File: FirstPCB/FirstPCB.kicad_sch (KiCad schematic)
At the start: 18 parts, among them J1 Conn_01x04_Socket, J2 Conn_01x08_Socket, U1 STM32G0B1KETx, U2 AMS1117-3.3

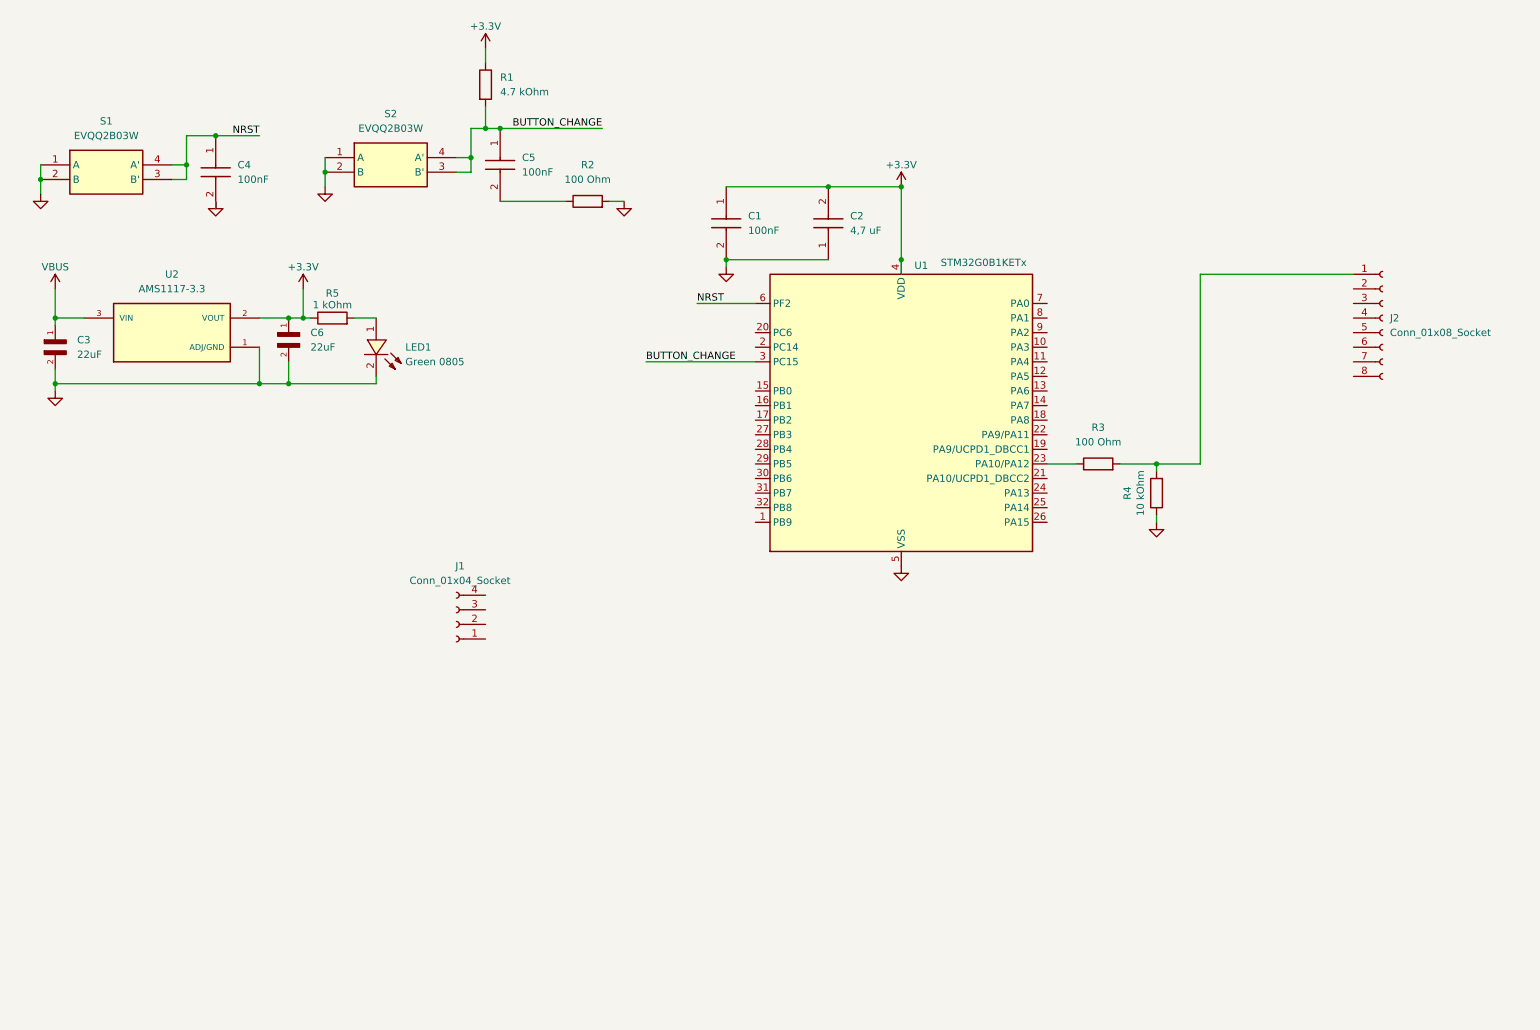
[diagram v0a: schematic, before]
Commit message: added sensor and schematic update
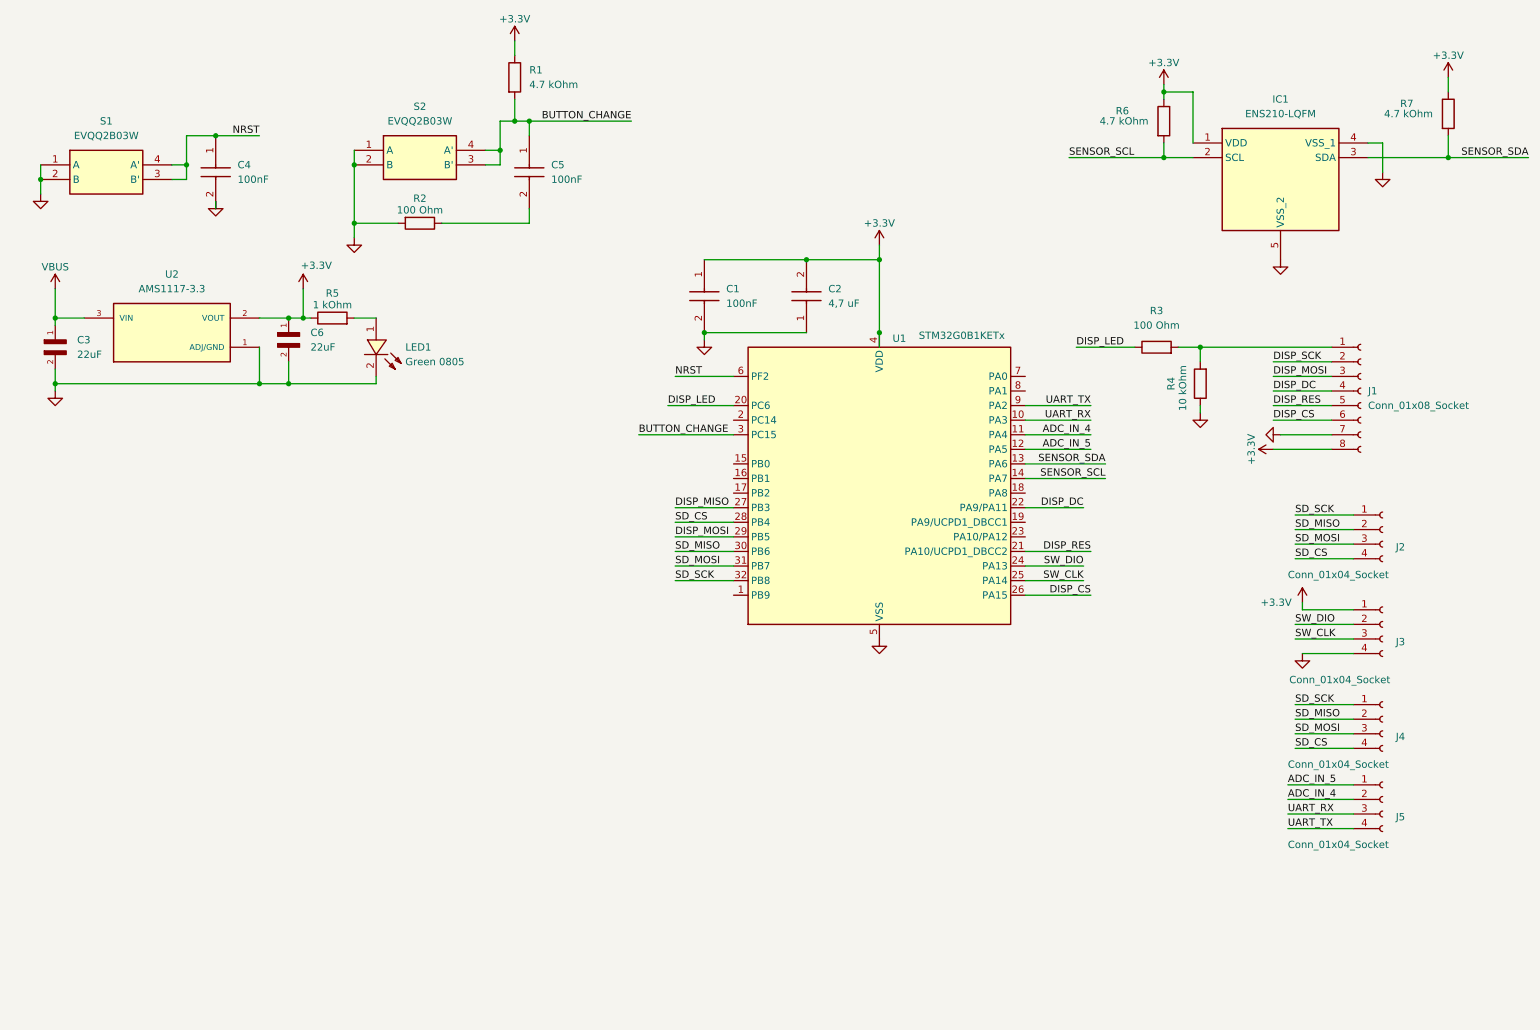
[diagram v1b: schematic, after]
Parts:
- added IC1: ENS210-LQFM, SON95P200X200X80-5N, symbol SamacSys_Parts:ENS210-LQFM
- added J3, J4, J5: Conn_01x04_Socket, Connector_PinSocket_2.54mm:PinSocket_1x04_P2.54mm_Vertical, symbol Connector:Conn_01x04_Socket
- added R6, R7: 4.7 kOhm, Resistor_SMD:R_0805_2012Metric, symbol Device:R
- renumbered J2 to J1, J1 to J2
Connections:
- net +3.3V: now also J1.8 (Pin_8), IC1.1 (VDD), J3.1 (Pin_1), R6.1, R7.1
- net GND: now also J1.7 (Pin_7), IC1.4 (VSS_1), IC1.5 (VSS_2), J3.4 (Pin_4)
- net UART_RX: now reaches U1.10 (PA3)
- net UART_RX: now also J5.3 (Pin_3)
- net ADC_IN_4: now reaches U1.11 (PA4)
- net ADC_IN_4: now also J5.2 (Pin_2)
- net ADC_IN_5: now reaches U1.12 (PA5)
- net ADC_IN_5: now also J5.1 (Pin_1)
- net SENSOR_SDA: now reaches U1.13 (PA6)
- net SENSOR_SDA: now also IC1.3 (SDA), R7.2
- net SENSOR_SCL: now reaches U1.14 (PA7)
- net SENSOR_SCL: now also IC1.2 (SCL), R6.2
- net DISP_LED: now reaches U1.20 (PC6)
- net DISP_LED: now also R3.1
- net DISP_RES: now reaches U1.21 (PA10/UCPD1_DBCC2)
- net DISP_RES: now also J1.5 (Pin_5)
- net DISP_DC: now reaches U1.22 (PA9/PA11)
- net DISP_DC: now also J1.4 (Pin_4)
- net at U1.23 (PA10/PA12): no longer R3.1
- net SW_DIO: now reaches U1.24 (PA13)
- net SW_DIO: now also J3.2 (Pin_2)
- net SW_CLK: now reaches U1.25 (PA14)
- net SW_CLK: now also J3.3 (Pin_3)
- net DISP_CS: now reaches U1.26 (PA15)
- net DISP_CS: now also J1.6 (Pin_6)
- net DISP_MISO: now reaches U1.27 (PB3)
- net SD_CS: now reaches U1.28 (PB4)
- net SD_CS: now also J2.4 (Pin_4), J4.4 (Pin_4)
- net DISP_MOSI: now reaches U1.29 (PB5)
- net DISP_MOSI: now also J1.3 (Pin_3)
- net SD_MISO: now reaches U1.30 (PB6)
- net SD_MISO: now also J2.2 (Pin_2), J4.2 (Pin_2)
- net SD_MOSI: now reaches U1.31 (PB7)
- net SD_MOSI: now also J2.3 (Pin_3), J4.3 (Pin_3)
- net SD_SCK: now reaches U1.32 (PB8)
- net SD_SCK: now also J2.1 (Pin_1), J4.1 (Pin_1)
- net UART_TX: now reaches U1.9 (PA2)
- net UART_TX: now also J5.4 (Pin_4)
- net DISP_SCK: now reaches J1.2 (Pin_2)
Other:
- title: STM32->Display -> First PCB
- moved on the sheet: C1, C2, C5, J1, J2, R1, R2, R3, R4, S2, U1

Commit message: shematic finished
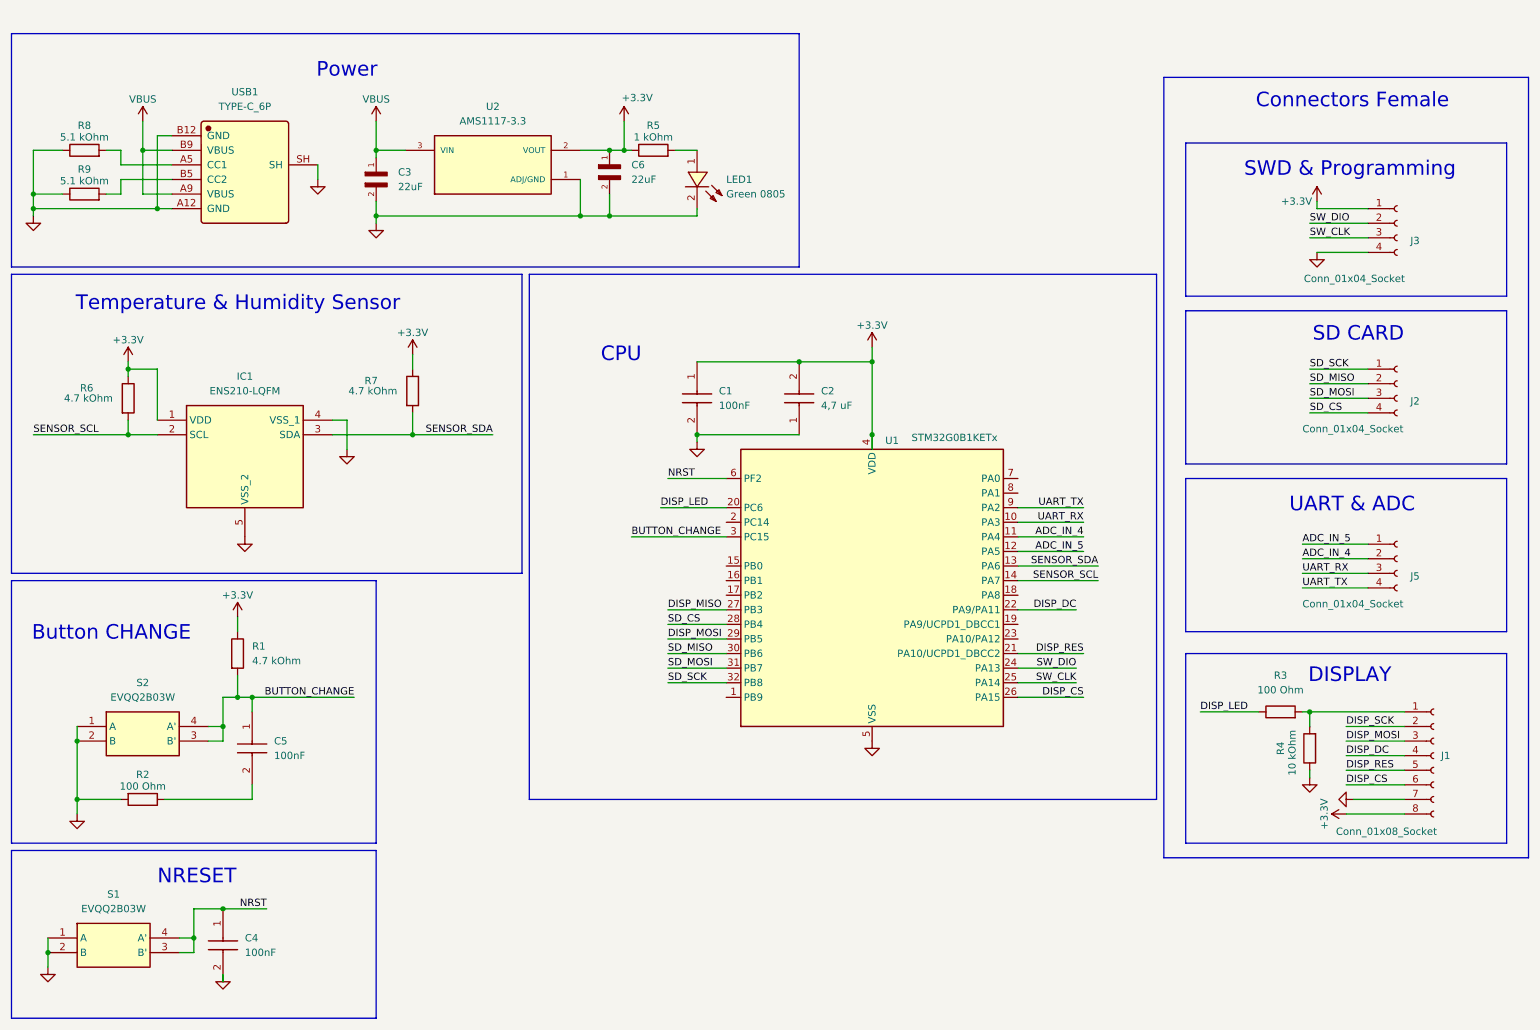
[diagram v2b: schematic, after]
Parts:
- removed J4: Conn_01x04_Socket, Connector_PinSocket_2.54mm:PinSocket_1x04_P2.54mm_Vertical, symbol Connector:Conn_01x04_Socket
- added R8, R9: 5.1 kOhm, Resistor_SMD:R_0805_2012Metric, symbol Device:R
- added USB1: TYPE-C_6P, Connector_USB:USB_C_Receptacle_GCT_USB4135-GF-A_6P_TopMnt_Horizontal, symbol JLCImport:TYPE-C_6P
- IC1: footprint SON95P200X200X80-5N -> SamacSys_Parts:SON95P200X200X80-5N
- LED1: footprint C2292:LED0805-R-RD -> CRG1206F470R:RESC3115X65N
- U2: footprint AMS1117-3.3:SOT229P700X180-4N -> Package_TO_SOT_SMD:SOT-223-3_TabPin2
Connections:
- net GND: now also R8.1, R9.1, USB1.A12 (GND), USB1.B12 (GND), USB1.SH
- net VBUS: now also USB1.A9 (VBUS), USB1.B9 (VBUS)
- new net: R9.2, USB1.B5 (CC2)
- new net: R8.2, USB1.A5 (CC1)
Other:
- note added: "Button CHANGE"
- note added: "CPU"
- note added: "Connectors Female"
- note added: "DISPLAY"
- note added: "NRESET"
- note added: "Power"
- note added: "SD CARD"
- note added: "SWD & Programming"
- note added: "Temperature & Humidity Sensor"
- note added: "UART & ADC"
- company: (none) -> Smart Avtomatic & Granitovich
- moved on the sheet: C1, C2, C3, C4, C5, C6, IC1, J1, J2, J3, J5, LED1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
